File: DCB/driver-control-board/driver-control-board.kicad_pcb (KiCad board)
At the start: 2 copper layers, 92.7 x 59.2 mm, 33 parts, among them J1 Conn_01x05, J2 Conn_01x14, J3 Conn_01x08, J4 Conn_01x23, U1 STM32F413CGUx, U2 LD1117S33TR_SOT223, U3 R-78B5.0-2.0, U4 MCP2551-I-SN, Y1 Crystal

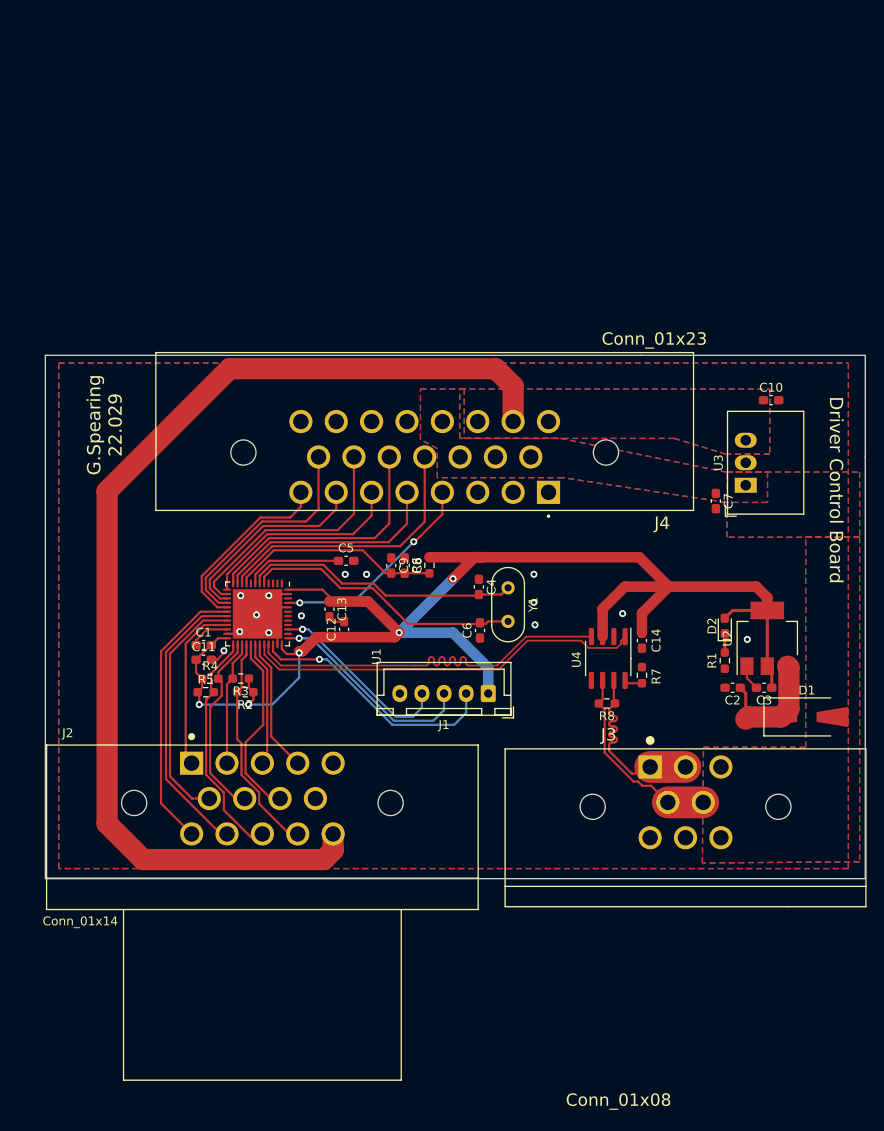
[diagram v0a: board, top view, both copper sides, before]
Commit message: DRC and Labeling Complete
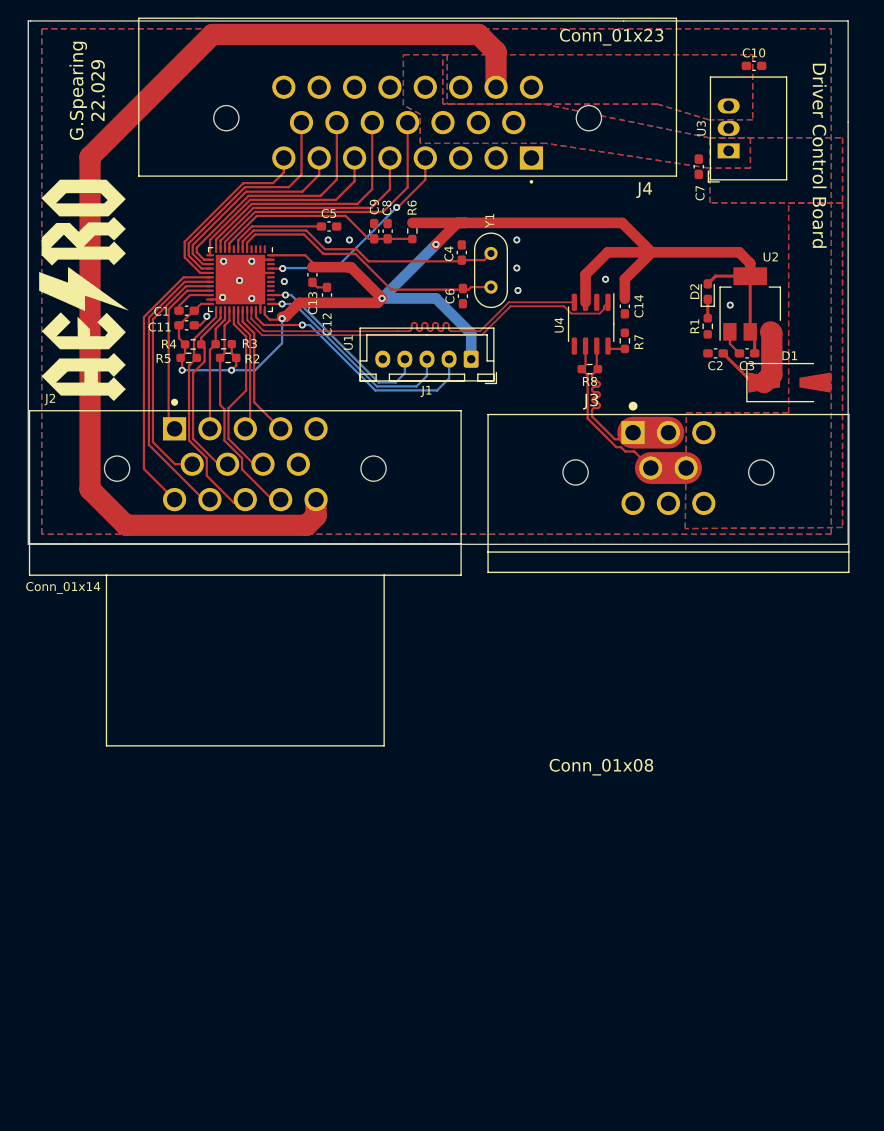
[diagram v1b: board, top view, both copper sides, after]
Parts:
- added G***: LOGO, AERO_Footprints:AERO_Logo_25x10mm, F.Cu at (99.9, 97.8)
- moved C4 37.9 mm to (142.6, 93.5)
- moved D1 37.9 mm to (179.7, 108.2)
- moved R8 37.9 mm to (157.1, 106.7)
- moved C7 37.9 mm to (169.4, 83.8)
- moved U4 37.9 mm to (157.2, 101.6)
- moved C1 37.9 mm to (111.5, 100.1)
- moved C10 37.9 mm to (175.6, 72.4)
- moved C11 37.9 mm to (111.5, 101.8)
- moved C12 37.9 mm to (127.4, 98.3)
- moved C13 37.9 mm to (125.7, 96.1)
- moved C8 37.9 mm to (134.2, 91.1)
- moved C9 37.9 mm to (132.7, 91.1)
- moved D2 37.9 mm to (170.4, 98.0)
- moved J1 37.9 mm to (143.7, 105.6)
- moved J2 37.9 mm to (118.1, 117.5)
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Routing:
- net Net-(C2-Pad1): track 14.1 -> 12.1 mm
